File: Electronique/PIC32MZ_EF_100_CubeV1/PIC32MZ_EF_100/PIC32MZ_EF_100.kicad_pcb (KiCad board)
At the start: 2 copper layers, 95.2 x 95.2 mm, 86 parts, among them J1001 Conn_02x20_Odd_Even, J1002 Conn_02x20_Odd_Even, J1003 Conn_01x04, J1004 USB_B_Mini, J1005 RJ12, J2001 Conn_02x05_Top_Bottom, J2002 Conn_02x05_Top_Bottom, Q2001 BC817, Q2002 BC817, Q3001 2N7002, Q3002 2N7002, Q3003 2N7002, SW1001 SW_Push, U2001 PCF8563T, U2002 MCP1501-SN, U3001 24LC1025, U3002 LM75A, U3003 SAA1064T, U3004 PIC32MZ2048EF100, X3001 32.768KHz, Y2001 24Mhz, Y2003 Crystal

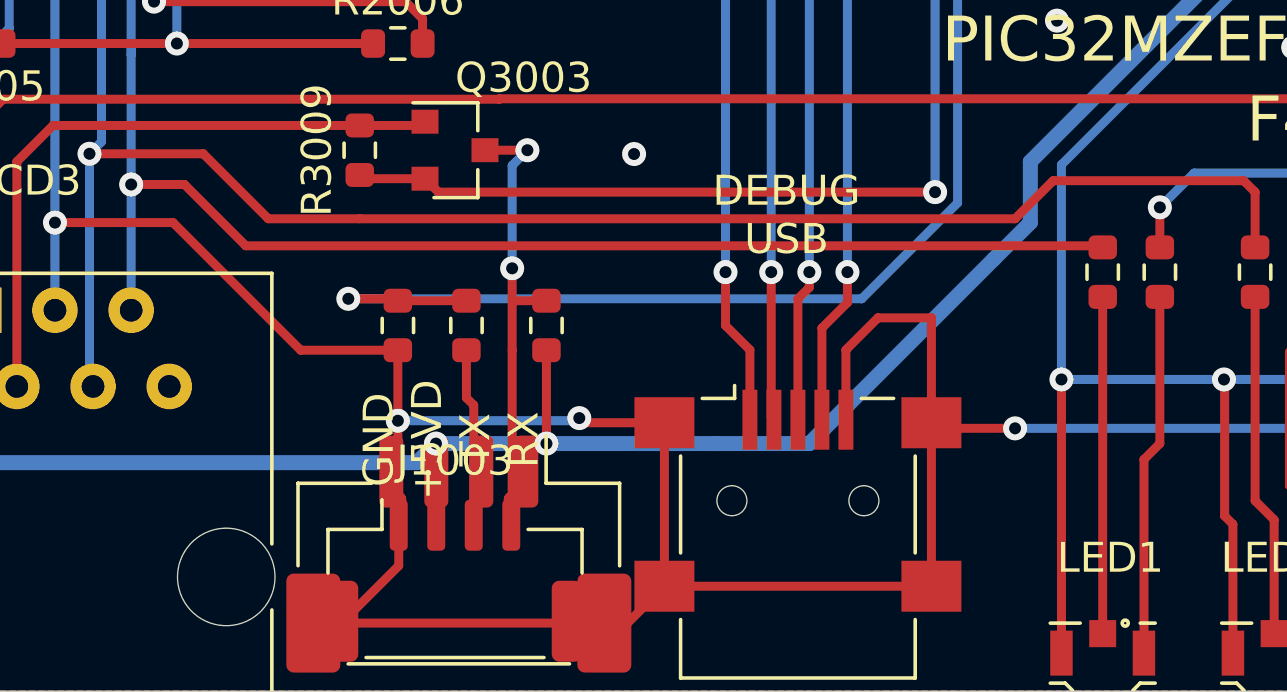
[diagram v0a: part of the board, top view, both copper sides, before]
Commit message: MAJ init
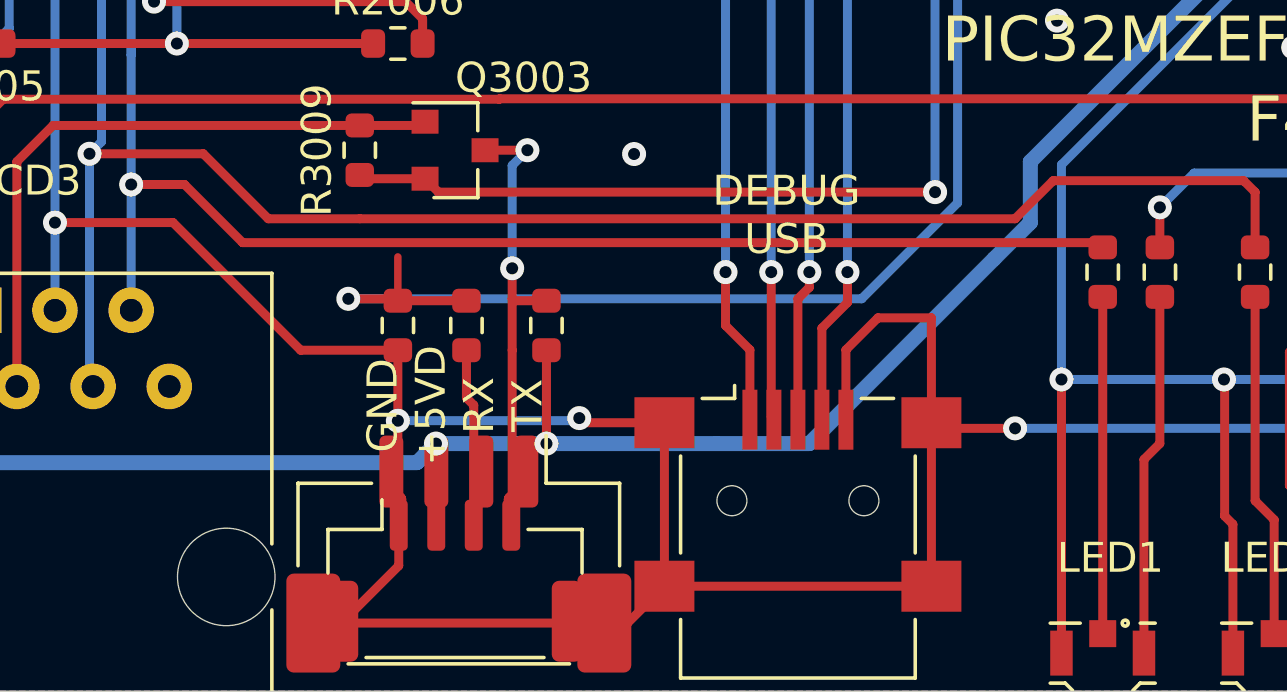
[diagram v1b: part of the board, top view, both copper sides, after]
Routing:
- net Net-(R3007-Pad2): track 85.8 -> 87.2 mm
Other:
- board text added: "GND +5VD RX TX"
- board text removed: "GND +5VD TX RX"

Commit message: Test INPUT CAPTURE 2
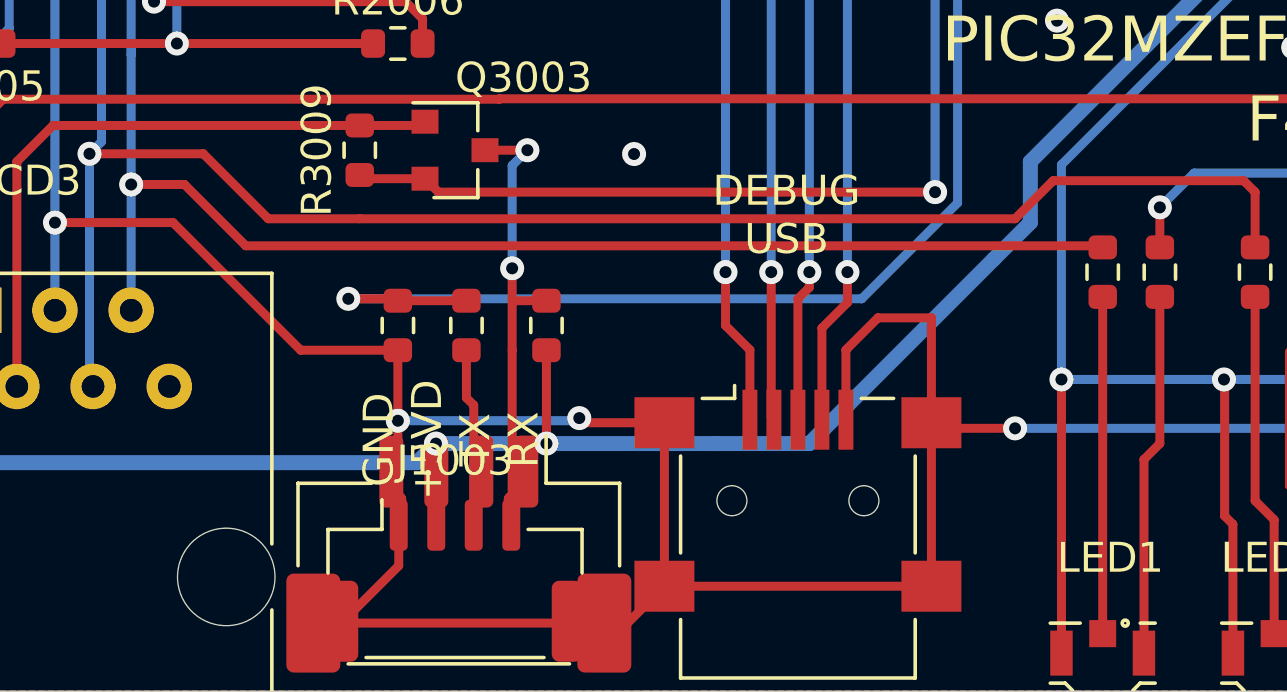
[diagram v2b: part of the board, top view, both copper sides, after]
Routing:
- net Net-(R3007-Pad2): track 87.2 -> 85.8 mm
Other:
- board text added: "GND +5VD TX RX"
- board text removed: "GND +5VD RX TX"
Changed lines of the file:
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@@
     (thickness 1.6)
     (drawings 84)
-    (tracks 1970)
+    (tracks 1969)
     (zones 0)
     (modules 86)
@@
   (layers
     (0 F.Cu signal)
-    (31 B.Cu signal)
+    (31 B.Cu signal hide)
     (32 B.Adhes user hide)
     (33 F.Adhes user)
@@
     (tags "connector JST GH top entry")
     (attr smd)
-    (fp_text reference J1003 (at 0 -4) (layer F.SilkS) hide
+    (fp_text reference J1003 (at 0 -4) (layer F.SilkS)
       (effects (font (size 1 1) (thickness 0.15)))
     )
@@
     (effects (font (size 1 1) (thickness 0.15)))
   )
-  (gr_text "GND\n+5VD\nRX\nTX" (at 132.715 132.715 90) (layer F.SilkS)
+  (gr_text "GND\n+5VD\nTX\nRX" (at 132.588 133.858 90) (layer F.SilkS)
     (effects (font (size 1 1) (thickness 0.15)))
   )
@@
   (segment (start 121.92 125.349) (end 121.92 121.031) (width 0.3) (layer B.Cu) (net 73))
   (segment (start 121.92 129.54) (end 121.92 125.349) (width 0.3) (layer B.Cu) (net 73) (status 10))
+  (segment (start 121.92 125.349) (end 123.698 125.349) (width 0.3) (layer F.Cu) (net 73))
+  (segment (start 125.741998 127.392998) (end 154.252998 127.392998) (width 0.3) (layer F.Cu) (net 73) (status 20))
+  (segment (start 123.698 125.349) (end 125.741998 127.392998) (width 0.3) (layer F.Cu) (net 73))
+  (segment (start 154.252998 127.392998) (end 154.305 127.445) (width 0.3) (layer F.Cu) (net 73) (status 30))
   (via (at 126.78299 76.036013) (size 0.8) (drill 0.4) (layers F.Cu B.Cu) (net 73))
   (segment (start 121.92 80.899003) (end 126.382991 76.436012) (width 0.3) (layer B.Cu) (net 73))
@@
   (segment (start 147.588425 74.915575) (end 147.503827 74.830977) (width 0.3) (layer F.Cu) (net 73))
   (segment (start 147.503827 74.830977) (end 127.988026 74.830977) (width 0.3) (layer F.Cu) (net 73))
-  (segment (start 121.92 125.349) (end 123.698 125.349) (width 0.3) (layer F.Cu) (net 73))
-  (segment (start 123.698 125.349) (end 125.635969 127.286969) (width 0.3) (layer F.Cu) (net 73))
-  (segment (start 125.635969 127.286969) (end 154.146969 127.286969) (width 0.3) (layer F.Cu) (net 73))
-  (segment (start 154.146969 127.286969) (end 154.305 127.445) (width 0.3) (layer F.Cu) (net 73))
   (segment (start 149.089154 76.294435) (end 149.065435 76.294435) (width 0.25) (layer F.Cu) (net 74) (status 30))
   (segment (start 148.209 75.438) (end 148.082 75.438) (width 0.25) (layer F.Cu) (net 74))
@@
   (segment (start 172.997967 84.939033) (end 172.997967 90.273033) (width 0.3) (layer B.Cu) (net 83))
   (segment (start 173.482 84.455) (end 172.997967 84.939033) (width 0.3) (layer B.Cu) (net 83))
-  (segment (start 130.81 129.223) (end 130.81 127.761979) (width 0.25) (layer F.Cu) (net 83))
   (segment (start 124.333 62.229) (end 124.332 62.23) (width 0.5) (layer F.Cu) (net 84) (status 30))
   (segment (start 124.333 59.69) (end 124.333 62.229) (width 0.5) (layer F.Cu) (net 84) (status 30))
